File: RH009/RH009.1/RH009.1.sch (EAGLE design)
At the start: 22 parts, among them Q2 BSS138, Q3 BSS138

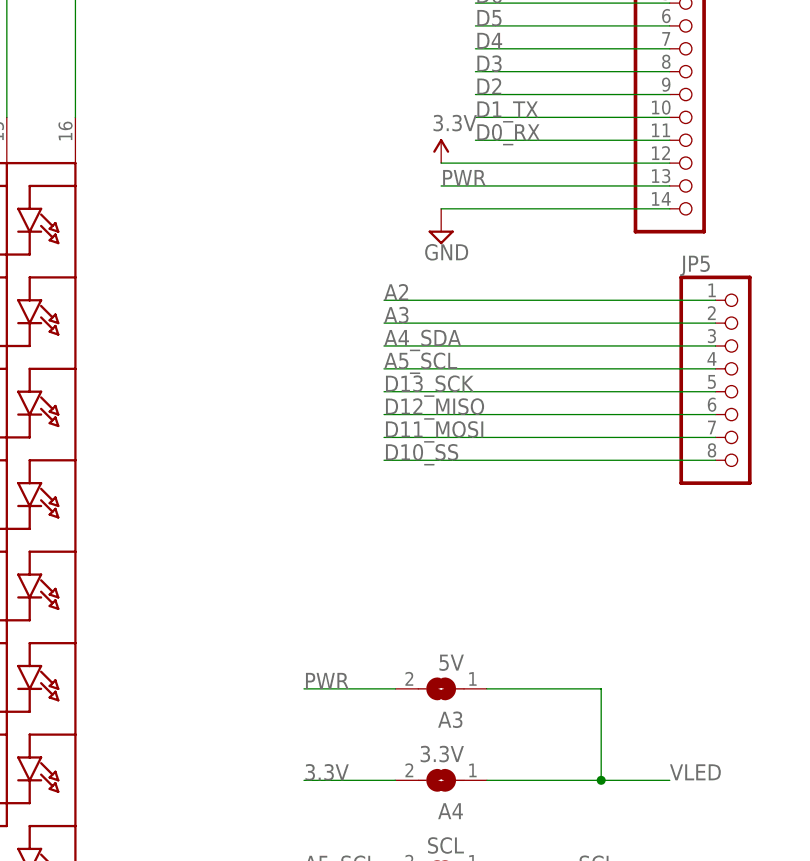
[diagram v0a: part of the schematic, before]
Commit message: Minor fixes
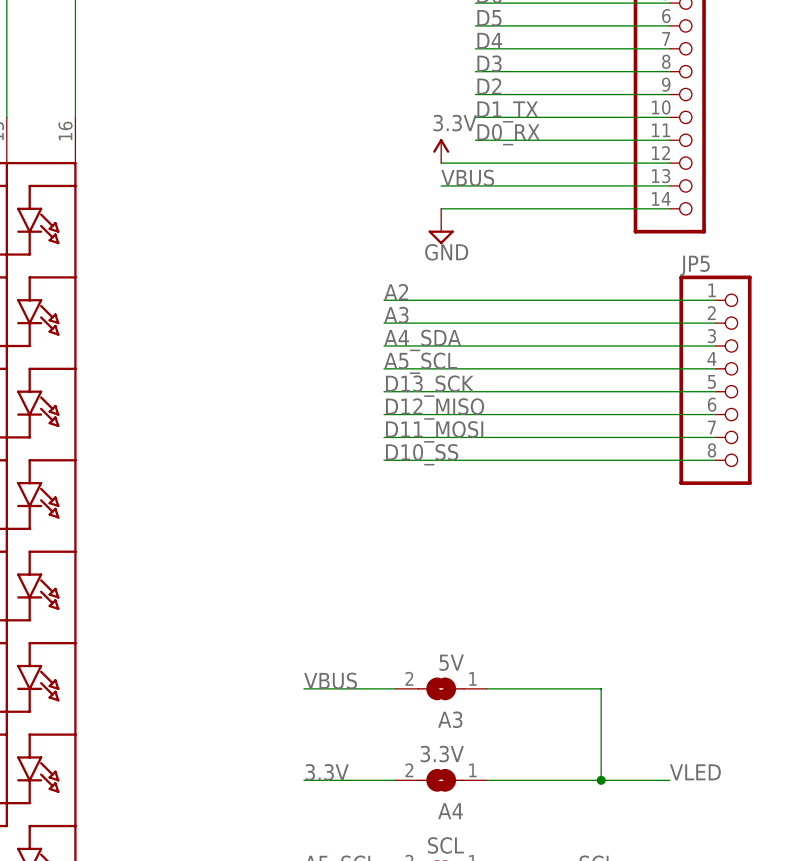
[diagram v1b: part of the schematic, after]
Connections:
- removed net PWR: A3.2, JP3.13
- net VBUS: now also A3.2, JP3.13
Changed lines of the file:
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@@
-</segment>
-</net>
-<net name="PWR" class="1">
-<segment>
-<wire x1="215.9" y1="134.62" x2="241.3" y2="134.62" width="0.1524" layer="91"/>
-<label x="215.9" y="134.62" size="1.778" layer="95"/>
-<pinref part="JP3" gate="A" pin="13"/>
-</segment>
-<segment>
-<pinref part="A3" gate="1" pin="2"/>
-<wire x1="210.82" y1="78.74" x2="200.66" y2="78.74" width="0.1524" layer="91"/>
-<label x="200.66" y="78.74" size="1.778" layer="95"/>
 </segment>
 </net>
@@
 <label x="140.97" y="33.02" size="1.778" layer="95"/>
 </segment>
+<segment>
+<wire x1="215.9" y1="134.62" x2="241.3" y2="134.62" width="0.1524" layer="91"/>
+<label x="215.9" y="134.62" size="1.778" layer="95"/>
+<pinref part="JP3" gate="A" pin="13"/>
+</segment>
+<segment>
+<pinref part="A3" gate="1" pin="2"/>
+<wire x1="210.82" y1="78.74" x2="200.66" y2="78.74" width="0.1524" layer="91"/>
+<label x="200.66" y="78.74" size="1.778" layer="95"/>
+</segment>
 </net>

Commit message: Board 9.1 finished
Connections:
- removed net VCC: Q2.G, Q3.G, R3.1, R5.1
- net 3.3V: now also Q2.G, Q3.G, R3.1, R5.1
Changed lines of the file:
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@@
 <label x="200.66" y="68.58" size="1.778" layer="95"/>
+</segment>
+<segment>
+<wire x1="77.47" y1="27.94" x2="77.47" y2="30.48" width="0.1524" layer="91"/>
+<wire x1="85.09" y1="22.86" x2="85.09" y2="30.48" width="0.1524" layer="91"/>
+<wire x1="85.09" y1="30.48" x2="77.47" y2="30.48" width="0.1524" layer="91"/>
+<junction x="77.47" y="30.48"/>
+<pinref part="R3" gate="G$1" pin="1"/>
+<pinref part="Q2" gate="G$1" pin="G"/>
+<pinref part="P+2" gate="1" pin="VCC"/>
+<wire x1="77.47" y1="35.56" x2="77.47" y2="30.48" width="0.1524" layer="91"/>
+</segment>
+<segment>
+<wire x1="125.73" y1="27.94" x2="125.73" y2="30.48" width="0.1524" layer="91"/>
+<wire x1="133.35" y1="22.86" x2="133.35" y2="30.48" width="0.1524" layer="91"/>
+<wire x1="133.35" y1="30.48" x2="125.73" y2="30.48" width="0.1524" layer="91"/>
+<junction x="125.73" y="30.48"/>
+<pinref part="R5" gate="G$1" pin="1"/>
+<pinref part="Q3" gate="G$1" pin="G"/>
+<pinref part="P+3" gate="1" pin="VCC"/>
+<wire x1="125.73" y1="35.56" x2="125.73" y2="30.48" width="0.1524" layer="91"/>
 </segment>
 </net>
@@
 </segment>
 </net>
-<net name="VCC" class="0">
-<segment>
-<wire x1="77.47" y1="27.94" x2="77.47" y2="30.48" width="0.1524" layer="91"/>
-<wire x1="85.09" y1="22.86" x2="85.09" y2="30.48" width="0.1524" layer="91"/>
-<wire x1="85.09" y1="30.48" x2="77.47" y2="30.48" width="0.1524" layer="91"/>
-<junction x="77.47" y="30.48"/>
-<pinref part="R3" gate="G$1" pin="1"/>
-<pinref part="Q2" gate="G$1" pin="G"/>
-<pinref part="P+2" gate="1" pin="VCC"/>
-<wire x1="77.47" y1="35.56" x2="77.47" y2="30.48" width="0.1524" layer="91"/>
-</segment>
-<segment>
-<wire x1="125.73" y1="27.94" x2="125.73" y2="30.48" width="0.1524" layer="91"/>
-<wire x1="133.35" y1="22.86" x2="133.35" y2="30.48" width="0.1524" layer="91"/>
-<wire x1="133.35" y1="30.48" x2="125.73" y2="30.48" width="0.1524" layer="91"/>
-<junction x="125.73" y="30.48"/>
-<pinref part="R5" gate="G$1" pin="1"/>
-<pinref part="Q3" gate="G$1" pin="G"/>
-<pinref part="P+3" gate="1" pin="VCC"/>
-<wire x1="125.73" y1="35.56" x2="125.73" y2="30.48" width="0.1524" layer="91"/>
-</segment>
-</net>
